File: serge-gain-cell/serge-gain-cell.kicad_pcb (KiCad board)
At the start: 2 copper layers, 40.5 x 28 mm, 20 parts, among them J1 Conn_01x08_Male, Q1 2N3906, Q2 2N3906, Q3 2N3904, Q4 2N3904, U1 LF353

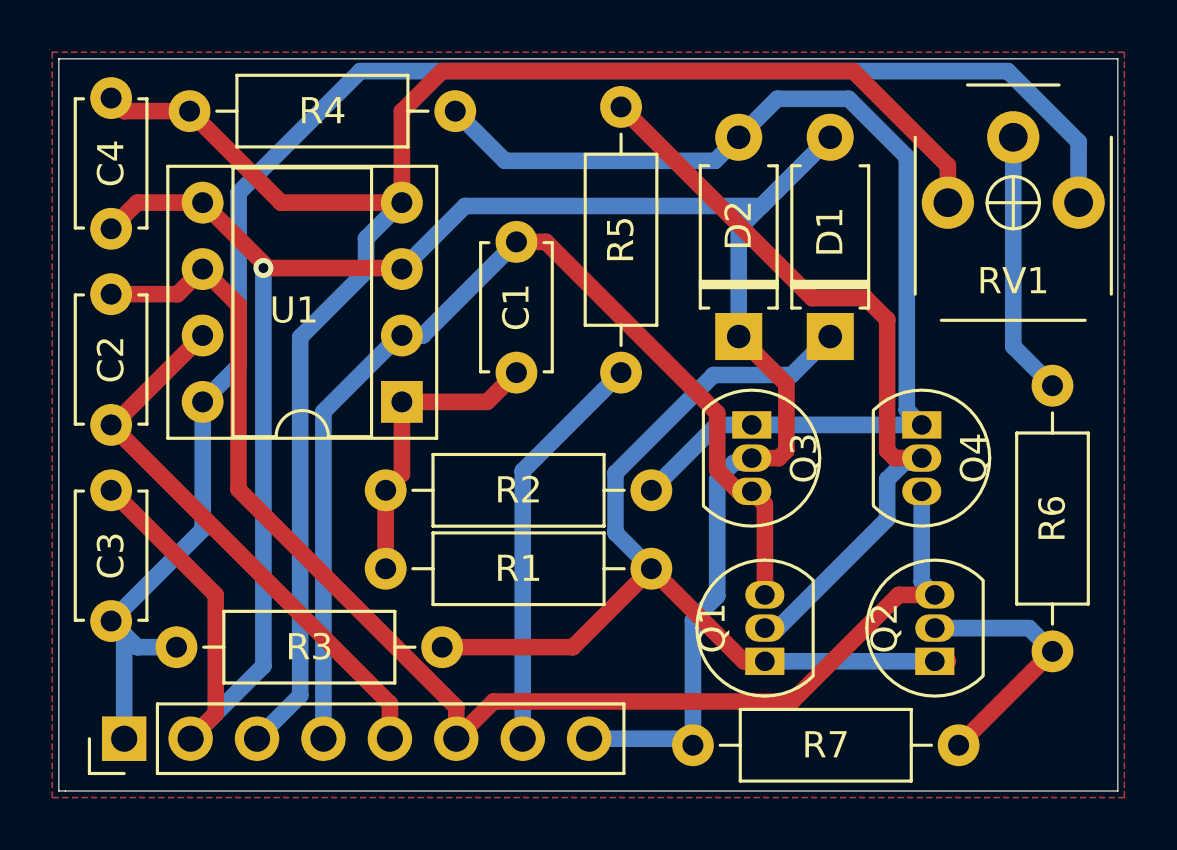
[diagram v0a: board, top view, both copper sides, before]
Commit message: Updating ordered boards
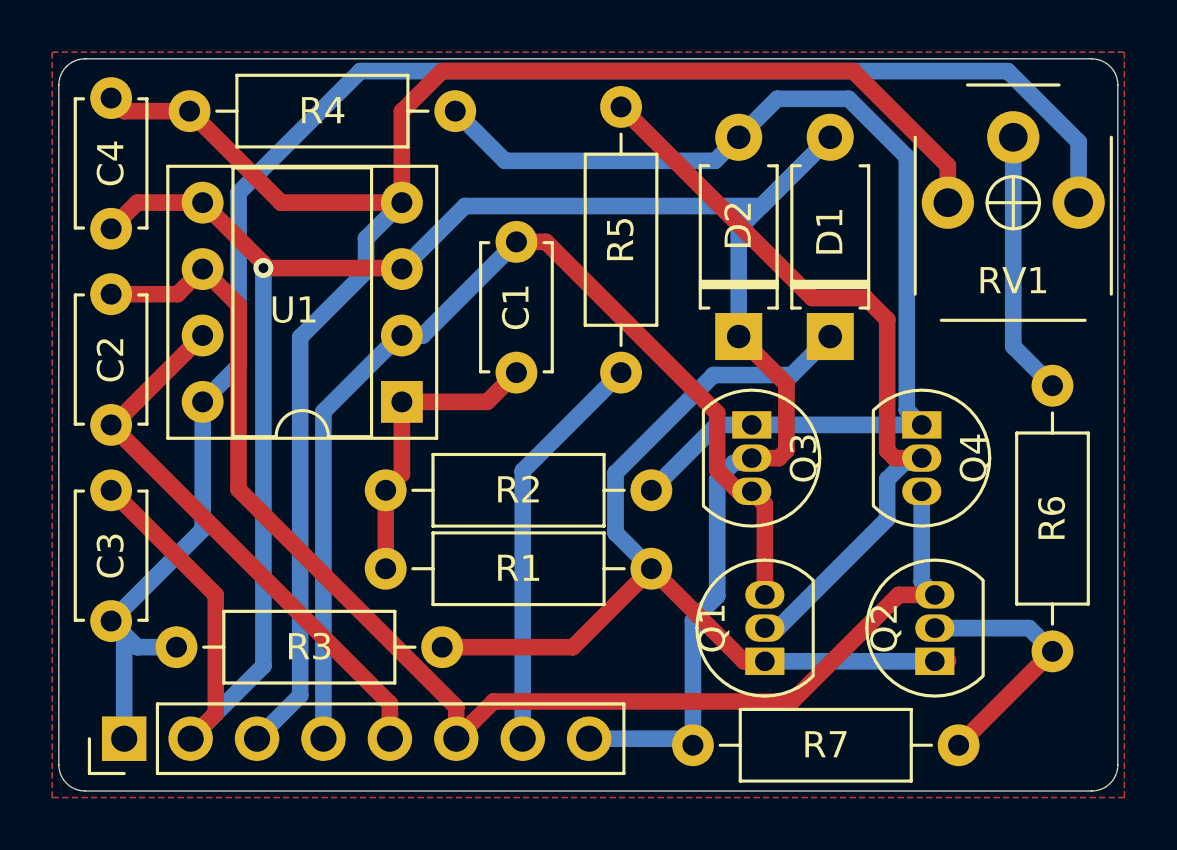
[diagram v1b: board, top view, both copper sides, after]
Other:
- outline, holes or cut-outs redrawn
- rule pad_to_mask_clearance: 0.0508 -> 0
